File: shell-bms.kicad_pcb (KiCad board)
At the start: 4 copper layers, 128.2 x 122.2 mm, 196 parts, among them J1 Conn_01x20, J10 Conn_01x05, J11 USB_C_Receptacle_USB2.0_16P, J13 OUTSIDE LED, J2 Conn_01x20, J3 Conn_01x04, J5 USB_C_Receptacle_USB2.0_16P, J6 Conn_01x02, J7 Conn_01x02, J8 Conn_01x02, J9 Conn_01x04, Q1 NPN, Q2 HY3610P, Q3 HY3610P, Q4 BC817, Q5 BC817, Q6 BC817, Q7 BC817, Q8 HY3610P, Q9 HY3610P, SW1 SW_Push, SW2 SW_Nidec_CAS-120A1, U1 BQ76952PFBR, U2 LM5017MR, U3 STM32G431C8Tx, U4 AP2204K-5.0, U5 CH340K, U6 XC6206 - 3V3, U7 ESP-WROOM-02, U8 TJA1051T, U9 CH340K, Y1 8MHz

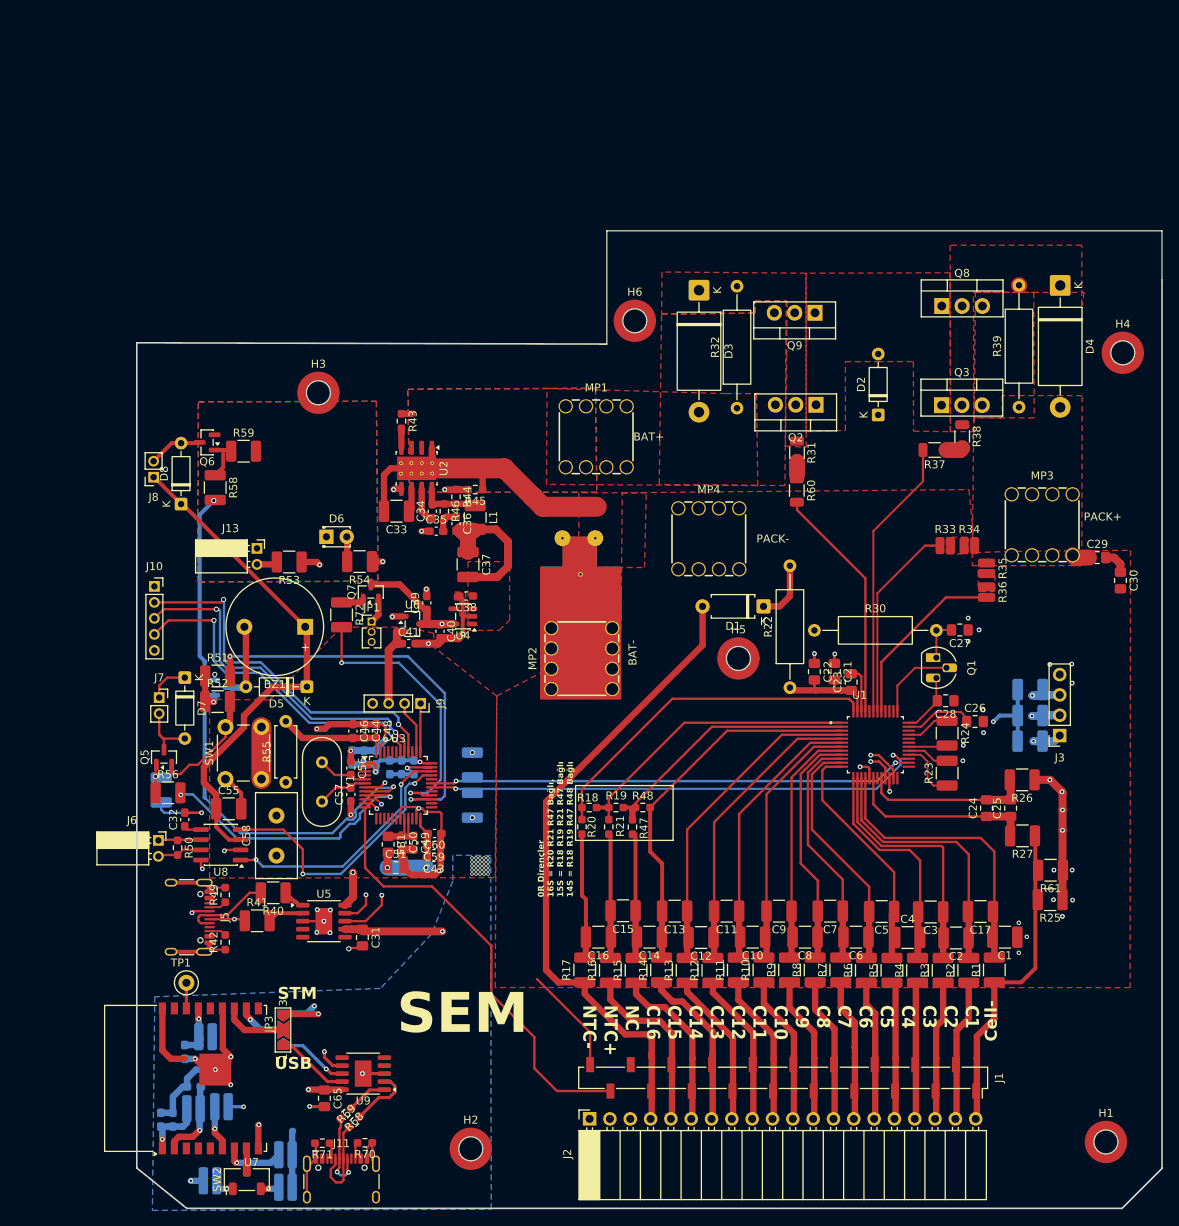
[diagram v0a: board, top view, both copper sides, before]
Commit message: BMS DONE IHOPE
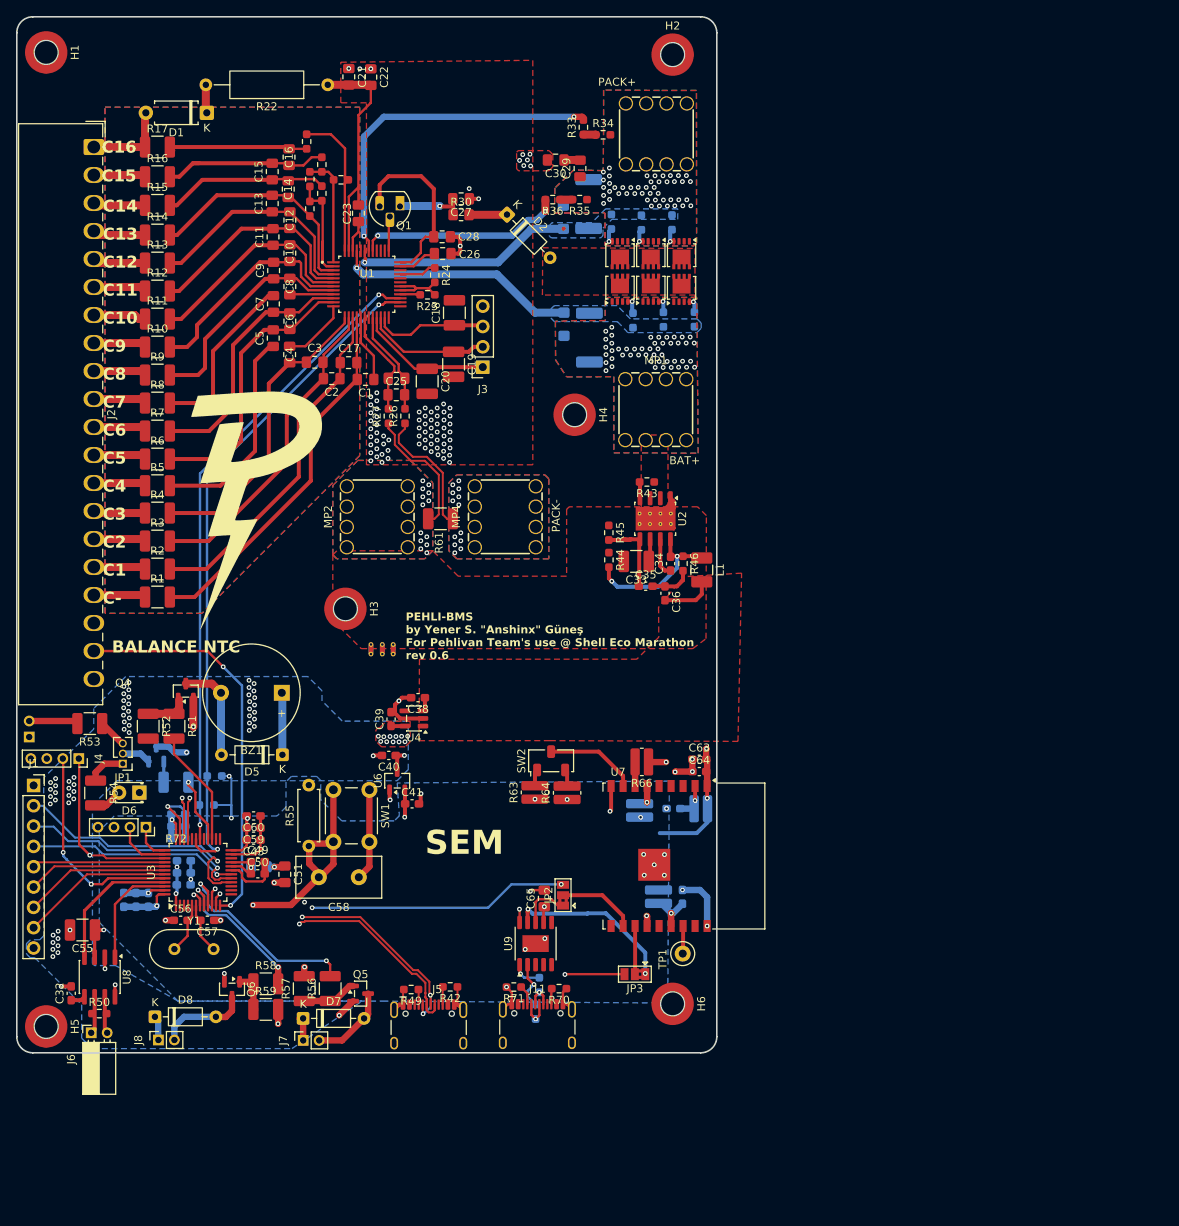
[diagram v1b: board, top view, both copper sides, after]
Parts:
- removed C31: 100nf, Capacitor_SMD:C_0805_2012Metric_Pad1.18x1.45mm_HandSolder
- removed C37: 47uF, Capacitor_SMD:C_1210_3225Metric_Pad1.33x2.70mm_HandSolder
- removed J10: Conn_01x05, Connector_PinSocket_2.00mm:PinSocket_1x05_P2.00mm_Vertical
- removed R40, R41: 22R, Resistor_SMD:R_1210_3225Metric_Pad1.30x2.65mm_HandSolder
- removed U5: CH340K, Package_SO:SSOP-10-1EP_3.9x4.9mm_P1mm_EP2.1x3.3mm
- added J4: Conn_01x04, Connector_PinSocket_2.00mm:PinSocket_1x04_P2.00mm_Vertical, F.Cu at (39.2, 113.7)
- added NT2: NetTie_2, NetTie:NetTie-2_THT_Pad0.3mm, F.Cu at (77.2, 99.5)
- added NT3: NetTie_2, NetTie:NetTie-2_THT_Pad0.3mm, F.Cu at (75.8, 99.5)
- added Q10: BUK7M27-80EX, Package_TO_SOT_SMD:LFPAK33, F.Cu at (110.7, 50.6)
- added Q11: BUK7M27-80EX, Package_TO_SOT_SMD:LFPAK33, F.Cu at (114.6, 50.6)
- added R73: 47, Resistor_SMD:R_0603_1608Metric_Pad0.98x0.95mm_HandSolder, B.Cu at (113.4, 46.7)
- C1, C10, C11, C12, C13, C14, C15, C16, C17, C2, C3, C4, C5, C6, C7, C8, C9: footprint Capacitor_SMD:C_1210_3225Metric_Pad1.33x2.70mm_HandSolder -> Capacitor_SMD:C_0805_2012Metric_Pad1.18x1.45mm_HandSolder
- C18, C19, C20, C63, C64, G***, Q4, R57, R63, R64, R66: moved to F.Cu
- C44, C46, C48, FB1, J13, Q7, R68, R69, R72: moved to B.Cu
- D3, D4: footprint Diode_THT:D_DO-201_P15.24mm_Horizontal -> Diode_SMD:D_SMF; moved to B.Cu
- J1: value Conn_01x20 -> Conn_01x09; footprint Connector_PinSocket_2.54mm:PinSocket_1x20_P2.54mm_Vertical_SMD_Pin1Right -> Connector_PinSocket_2.54mm:PinSocket_1x09_P2.54mm_Vertical
- J2: footprint Connector_PinSocket_2.54mm:PinSocket_1x20_P2.54mm_Horizontal -> Connector_Wago:Wago_734-180_1x20_P3.50mm_Horizontal
- JP2: footprint Jumper:SolderJumper-3_P2.0mm_Open_TrianglePad1.0x1.5mm_NumberLabels -> Jumper:SolderJumper-3_P1.3mm_Bridged2Bar12_Pad1.0x1.5mm; moved to F.Cu
- JP3: footprint Jumper:SolderJumper-3_P2.0mm_Open_TrianglePad1.0x1.5mm_NumberLabels -> Jumper:SolderJumper-3_P1.3mm_Bridged2Bar12_Pad1.0x1.5mm
- NT1: value NetTie_3_Tee -> NetTie_2; footprint NetTie:NetTie-3_THT_Pad0.3mm -> NetTie:NetTie-2_THT_Pad0.3mm
- Q2, Q3, Q8, Q9: value HY3610P -> BUK7M27-80EX; footprint Package_TO_SOT_THT:TO-220-3_Vertical -> Package_TO_SOT_SMD:LFPAK33
- R23, R24, R26, R27, R28, R29: footprint Resistor_SMD:R_1210_3225Metric_Pad1.30x2.65mm_HandSolder -> Resistor_SMD:R_0603_1608Metric_Pad0.98x0.95mm_HandSolder
- R25: value 1m -> 47; footprint Resistor_SMD:R_1210_3225Metric_Pad1.30x2.65mm_HandSolder -> Resistor_SMD:R_0603_1608Metric_Pad0.98x0.95mm_HandSolder; moved to B.Cu
- R30: value R -> 300; footprint Resistor_THT:R_Axial_DIN0309_L9.0mm_D3.2mm_P15.24mm_Horizontal -> Resistor_SMD:R_0805_2012Metric_Pad1.20x1.40mm_HandSolder
- R31, R37, R60: value 2k -> 47; footprint Resistor_SMD:R_1206_3216Metric -> Resistor_SMD:R_0603_1608Metric_Pad0.98x0.95mm_HandSolder; moved to B.Cu
- R32: footprint Resistor_THT:R_Axial_DIN0309_L9.0mm_D3.2mm_P15.24mm_Horizontal -> Resistor_SMD:R_2512_6332Metric_Pad1.40x3.35mm_HandSolder; moved to B.Cu
- R33, R34, R35, R36: footprint Resistor_SMD:R_0508_1220Metric_Pad1.12x2.15mm_HandSolder -> Resistor_SMD:R_0603_1608Metric_Pad0.98x0.95mm_HandSolder
- R38: value 2k -> 1M; footprint Resistor_SMD:R_1206_3216Metric -> Resistor_SMD:R_2512_6332Metric_Pad1.40x3.35mm_HandSolder; moved to B.Cu
- R39: value 1M -> 47; footprint Resistor_THT:R_Axial_DIN0309_L9.0mm_D3.2mm_P15.24mm_Horizontal -> Resistor_SMD:R_0603_1608Metric_Pad0.98x0.95mm_HandSolder; moved to B.Cu
- moved H1 190.0 mm to (35.2, 25.4), turned to -90 degrees
- moved H2 139.1 mm to (113.5, 25.7)
- moved J2 136.4 mm to (41.1, 37.3), turned to -90 degrees
- moved R17 115.9 mm to (49.1, 37.3), turned to 0 degrees
- moved R1 114.5 mm to (49.1, 93.5), turned to 0 degrees
- moved R16 114.2 mm to (49.1, 41.0), turned to 0 degrees
- moved R2 113.1 mm to (49.1, 90.0), turned to 0 degrees
- moved R15 112.8 mm to (49.1, 44.6), turned to 0 degrees
- moved R3 111.9 mm to (49.1, 86.5), turned to 0 degrees
- moved R14 111.4 mm to (49.1, 48.3), turned to 0 degrees
- moved R4 110.9 mm to (49.1, 83.0), turned to 0 degrees
- moved R13 110.5 mm to (49.1, 51.8), turned to 0 degrees
- moved R5 110.0 mm to (49.1, 79.6), turned to 0 degrees
- moved R12 109.7 mm to (49.1, 55.3), turned to 0 degrees
- moved R6 109.3 mm to (49.1, 76.3), turned to 0 degrees
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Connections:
- net /Data_Utils/RXD renamed /MCU/esp32/ESP_RX
- net /Data_Utils/TXD renamed /MCU/esp32/ESP_TX
- C29 pad 1: Net-(D4-A) -> /Protection/PACK+
- D1 pad 2: /ReaderIC/Balance-Input/B_16 -> /ReaderIC/Balance-Input/CI_16
- D3 pad 1: Net-(D3-K) -> /Protection/CHG_GATE
- D3 pad 2: /Protection/B_Pos -> /Protection/B_POS
- D4 pad 1: Net-(D4-K) -> /Protection/DSG_GATE
- D4 pad 2: Net-(D4-A) -> /Protection/PACK+
- J1 pad 1: /ReaderIC/Balance-Input/B_0 -> GND
- J1 pad 2: /ReaderIC/Balance-Input/B_1 -> /Data_Utils/PB0
- J1 pad 3: /ReaderIC/Balance-Input/B_2 -> /Data_Utils/PB1
- J1 pad 4: /ReaderIC/Balance-Input/B_3 -> /Data_Utils/PB2
- J1 pad 5: /ReaderIC/Balance-Input/B_4 -> /Data_Utils/PB3
- J1 pad 6: /ReaderIC/Balance-Input/B_5 -> /Data_Utils/PB4
- J1 pad 7: /ReaderIC/Balance-Input/B_6 -> /Data_Utils/PB5
- J1 pad 8: /ReaderIC/Balance-Input/B_7 -> /Data_Utils/PB6
- J1 pad 9: /ReaderIC/Balance-Input/B_8 -> +5V
- J2 pad 1: /ReaderIC/Balance-Input/B_0 -> /ReaderIC/Balance-Input/CI_16
- J2 pad 10: /ReaderIC/Balance-Input/B_9 -> /ReaderIC/Balance-Input/CI_7
- J2 pad 11: /ReaderIC/Balance-Input/B_10 -> /ReaderIC/Balance-Input/CI_6
- J2 pad 12: /ReaderIC/Balance-Input/B_11 -> /ReaderIC/Balance-Input/CI_5
- J2 pad 13: /ReaderIC/Balance-Input/B_12 -> /ReaderIC/Balance-Input/CI_4
- J2 pad 14: /ReaderIC/Balance-Input/B_13 -> /ReaderIC/Balance-Input/CI_3
- J2 pad 15: /ReaderIC/Balance-Input/B_14 -> /ReaderIC/Balance-Input/CI_2
- J2 pad 16: /ReaderIC/Balance-Input/B_15 -> /ReaderIC/Balance-Input/CI_1
- J2 pad 17: /ReaderIC/Balance-Input/B_16 -> /ReaderIC/Balance-Input/CI_0
- J2 pad 19: unconnected-(J2-Pin_19-Pad19) -> /MCU/NTC
- J2 pad 2: /ReaderIC/Balance-Input/B_1 -> /ReaderIC/Balance-Input/CI_15
- J2 pad 20: unconnected-(J2-Pin_20-Pad20) -> GND
- J2 pad 3: /ReaderIC/Balance-Input/B_2 -> /ReaderIC/Balance-Input/CI_14
- J2 pad 4: /ReaderIC/Balance-Input/B_3 -> /ReaderIC/Balance-Input/CI_13
- J2 pad 5: /ReaderIC/Balance-Input/B_4 -> /ReaderIC/Balance-Input/CI_12
- J2 pad 6: /ReaderIC/Balance-Input/B_5 -> /ReaderIC/Balance-Input/CI_11
- J2 pad 7: /ReaderIC/Balance-Input/B_6 -> /ReaderIC/Balance-Input/CI_10
- J2 pad 8: /ReaderIC/Balance-Input/B_7 -> /ReaderIC/Balance-Input/CI_9
- J2 pad 9: /ReaderIC/Balance-Input/B_8 -> /ReaderIC/Balance-Input/CI_8
- J5 pad A6: Net-(J5-D+-PadA6) -> /Data_Utils/USB+
- J5 pad A7: Net-(J5-D--PadA7) -> /Data_Utils/USB-
- J5 pad B6: Net-(J5-D+-PadA6) -> /Data_Utils/USB+
- J5 pad B7: Net-(J5-D--PadA7) -> /Data_Utils/USB-
- MP1 pad 1: /Protection/B_Pos -> /Protection/B_POS
- MP1 pad 2: /Protection/B_Pos -> /Protection/B_POS
- MP1 pad 3: /Protection/B_Pos -> /Protection/B_POS
- MP1 pad 4: /Protection/B_Pos -> /Protection/B_POS
- MP1 pad 5: /Protection/B_Pos -> /Protection/B_POS
- MP1 pad 6: /Protection/B_Pos -> /Protection/B_POS
- MP1 pad 7: /Protection/B_Pos -> /Protection/B_POS
- MP1 pad 8: /Protection/B_Pos -> /Protection/B_POS
- MP2 pad 1: Net-(MP2-Pad1) -> GNDPWR
- MP2 pad 2: Net-(MP2-Pad1) -> GNDPWR
- MP2 pad 3: Net-(MP2-Pad1) -> GNDPWR
- MP2 pad 4: Net-(MP2-Pad1) -> GNDPWR
- MP2 pad 5: Net-(MP2-Pad1) -> GNDPWR
- MP2 pad 6: Net-(MP2-Pad1) -> GNDPWR
- MP2 pad 7: Net-(MP2-Pad1) -> GNDPWR
- MP2 pad 8: Net-(MP2-Pad1) -> GNDPWR
- MP3 pad 1: Net-(D4-A) -> /Protection/PACK+
- MP3 pad 2: Net-(D4-A) -> /Protection/PACK+
- MP3 pad 3: Net-(D4-A) -> /Protection/PACK+
- MP3 pad 4: Net-(D4-A) -> /Protection/PACK+
- MP3 pad 5: Net-(D4-A) -> /Protection/PACK+
- MP3 pad 6: Net-(D4-A) -> /Protection/PACK+
- MP3 pad 7: Net-(D4-A) -> /Protection/PACK+
- MP3 pad 8: Net-(D4-A) -> /Protection/PACK+
- NT1 pad 1: GND -> GNDPWR
- NT1 pad 2: GNDPWR -> GND
- Q2 pad 1: /Protection/CD -> /Protection/PACK+
- Q2 pad 2: Net-(D3-K) -> /Protection/PACK+
- Q2 pad 3: /Protection/B_Pos -> /Protection/PACK+
- Q3 pad 1: /Protection/CD -> /Protection/B_POS
- Q3 pad 2: Net-(D4-K) -> /Protection/B_POS
- Q3 pad 3: Net-(D4-A) -> /Protection/B_POS
- Q7 pad 2: Net-(JP1-A) -> Net-(JP1-C)
- Q8 pad 1: /Protection/CD -> /Protection/B_POS
- Q8 pad 2: Net-(D4-K) -> /Protection/B_POS
- Q8 pad 3: Net-(D4-A) -> /Protection/B_POS
- Q9 pad 1: /Protection/CD -> /Protection/B_POS
- Q9 pad 2: Net-(D3-K) -> /Protection/B_POS
- Q9 pad 3: /Protection/B_Pos -> /Protection/B_POS
- R1 pad 1: /ReaderIC/Balance-Input/B_0 -> /ReaderIC/Balance-Input/CI_0
- R10 pad 1: /ReaderIC/Balance-Input/B_9 -> /ReaderIC/Balance-Input/CI_9
- R11 pad 1: /ReaderIC/Balance-Input/B_10 -> /ReaderIC/Balance-Input/CI_10
- R12 pad 1: /ReaderIC/Balance-Input/B_11 -> /ReaderIC/Balance-Input/CI_11
- R13 pad 1: /ReaderIC/Balance-Input/B_12 -> /ReaderIC/Balance-Input/CI_12
- R14 pad 1: /ReaderIC/Balance-Input/B_13 -> /ReaderIC/Balance-Input/CI_13
- R15 pad 1: /ReaderIC/Balance-Input/B_14 -> /ReaderIC/Balance-Input/CI_14
- R16 pad 1: /ReaderIC/Balance-Input/B_15 -> /ReaderIC/Balance-Input/CI_15
- R17 pad 1: /ReaderIC/Balance-Input/B_16 -> /ReaderIC/Balance-Input/CI_16
- R2 pad 1: /ReaderIC/Balance-Input/B_1 -> /ReaderIC/Balance-Input/CI_1
- R25 pad 1: GNDPWR -> /Protection/CHG_GATE
- R25 pad 2: /ReaderIC/Balance-Input/B_0 -> Net-(Q8-G)
- R27 pad 1: /ReaderIC/Balance-Input/B_0 -> GNDPWR
- R28 pad 1: /MCU/IC_SDA -> +3V3
- R28 pad 2: +3V3 -> /MCU/IC_SCL
- R29 pad 1: +3V3 -> /MCU/IC_SDA
- R29 pad 2: /MCU/IC_SCL -> +3V3
- R3 pad 1: /ReaderIC/Balance-Input/B_2 -> /ReaderIC/Balance-Input/CI_2
- R31 pad 1: Net-(D3-K) -> /Protection/CHG_GATE
- R31 pad 2: Net-(R31-Pad2) -> Net-(Q3-G)
- R32 pad 1: /Protection/B_Pos -> /Protection/B_POS
- R32 pad 2: Net-(D3-K) -> /Protection/CHG_GATE
- R33 pad 1: /Protection/PACK -> Net-(R33-Pad1)
- R33 pad 2: Net-(R33-Pad2) -> /Protection/PACK
- R34 pad 1: Net-(R33-Pad2) -> Net-(R33-Pad1)
- R34 pad 2: Net-(D4-A) -> /Protection/PACK+
- R35 pad 1: Net-(D4-A) -> /Protection/PACK+
- R37 pad 1: Net-(R37-Pad1) -> /Protection/CHG_GATE
- R37 pad 2: /Protection/DSG -> Net-(Q9-G)
- R38 pad 1: Net-(D4-K) -> /Protection/PACK+
- R38 pad 2: Net-(R37-Pad1) -> /Protection/DSG_GATE
- R39 pad 1: Net-(D4-A) -> /Protection/DSG_GATE
- R39 pad 2: Net-(D4-K) -> Net-(Q2-G)
- R4 pad 1: /ReaderIC/Balance-Input/B_3 -> /ReaderIC/Balance-Input/CI_3
- R43 pad 1: /Protection/B_Pos -> /Protection/B_POS
- R5 pad 1: /ReaderIC/Balance-Input/B_4 -> /ReaderIC/Balance-Input/CI_4
- R53 pad 1: Net-(JP1-C) -> Net-(JP1-B)
- R54 pad 1: Net-(JP1-B) -> Net-(JP1-A)
- R6 pad 1: /ReaderIC/Balance-Input/B_5 -> /ReaderIC/Balance-Input/CI_5
- R60 pad 1: Net-(R31-Pad2) -> /Protection/DSG_GATE
- R60 pad 2: /Protection/CHG -> Net-(Q10-G)
- R61 pad 2: /ReaderIC/Balance-Input/B_0 -> GNDPWR
- R7 pad 1: /ReaderIC/Balance-Input/B_6 -> /ReaderIC/Balance-Input/CI_6
- R8 pad 1: /ReaderIC/Balance-Input/B_7 -> /ReaderIC/Balance-Input/CI_7
- R9 pad 1: /ReaderIC/Balance-Input/B_8 -> /ReaderIC/Balance-Input/CI_8
- U1 pad 43: /Protection/DSG -> /Protection/DSG_GATE
- U1 pad 45: /Protection/CHG -> /Protection/CHG_GATE
- U2 pad 2: /Protection/B_Pos -> /Protection/B_POS
- U2 pad 3: /Protection/B_Pos -> /Protection/B_POS
- U3 pad 16: unconnected-(U3-PB0-Pad16) -> /Data_Utils/PB0
- U3 pad 17: unconnected-(U3-PB1-Pad17) -> /Data_Utils/PB1
- U3 pad 18: unconnected-(U3-PB2-Pad18) -> /Data_Utils/PB2
- U3 pad 33: /Data_Utils/CAN_RX -> /Data_Utils/USB+
- U3 pad 34: /Data_Utils/CAN_TX -> /Data_Utils/USB-
- U3 pad 39: unconnected-(U3-PA15-Pad39) -> /MCU/I2C_SCL
- U3 pad 43: unconnected-(U3-PB6-Pad43) -> /Data_Utils/PB6
- U3 pad 44: unconnected-(U3-PB7-Pad44) -> /MCU/I2C_SDA
- U3 pad 45: unconnected-(U3-PB8-Pad45) -> /Data_Utils/CAN_RX
- U3 pad 46: unconnected-(U3-PB9-Pad46) -> /Data_Utils/CAN_TX
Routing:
- net +5V: track 123.9 -> 30.1 mm, vias 1 -> 68
- net GND: track 188.2 -> 105.7 mm, vias 30 -> 38
- net /ReaderIC/Balance-Input/B_16: track 81.9 -> 0.00 mm
- net /Data_Utils/USB-: track 4.54 -> 60.3 mm, vias 0 -> 4
- net /Data_Utils/USB+: track 2.79 -> 57.7 mm, vias 0 -> 2
- net /Data_Utils/FAN2: track 70.7 -> 19.4 mm
- net /ReaderIC/Balance-Input/B_0: track 40.9 -> 0.00 mm
- net +3V3: track 122.2 -> 82.5 mm, vias 36 -> 14
- net /Data_Utils/BUZZER: track 51.0 -> 14.5 mm, vias 2 -> 0
- net /Protection/DSG: track 35.2 -> 0.00 mm
- net /Data_Utils/PB0: track 0.00 -> 32.6 mm, vias 0 -> 1
- net GNDPWR: track 95.4 -> 63.5 mm, vias 26 -> 103
- net /Protection/CHG_GATE: track 0.00 -> 30.4 mm, vias 0 -> 1
- net /Protection/CHG: track 30.1 -> 0.00 mm
- net /Data_Utils/PB3: track 46.0 -> 16.6 mm, vias 2 -> 0
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- added copper zone on B.Cu, net (none)
- added copper zone on F.Cu, net (none)
- added copper zone on In1.Cu, net (none)
- added copper zone on In2.Cu, net (none)
- added copper zone on In2.Cu, net +3V3
- added copper zone on B.Cu, net +5V
- added copper zone on F.Cu, net +5V
- added copper zone on In2.Cu, net +5V
- added copper zone on B.Cu, net /Protection/B_POS
- added copper zone on F.Cu, net /Protection/B_POS
- added copper zone on In1.Cu, net /Protection/B_POS
- added copper zone on In2.Cu, net /Protection/B_POS
- added copper zone on In1.Cu, net /Protection/CD
- added copper zone on In2.Cu, net /Protection/CD
- added copper zone on B.Cu, net /Protection/CHG_GATE
- added copper zone on B.Cu, net /Protection/DSG_GATE
- added copper zone on B.Cu, net /Protection/PACK+
- added copper zone on F.Cu, net /Protection/PACK+
- added copper zone on In1.Cu, net /Protection/PACK+
- added copper zone on In2.Cu, net /Protection/PACK+
- added copper zone on B.Cu, net GNDPWR
- added copper zone on In2.Cu, net GNDPWR
- removed copper zone on F.Cu, net +3V3
- removed copper zone on B.Cu, net /Protection/B_Pos
- removed copper zone on F.Cu, net /Protection/B_Pos
- removed copper zone on In1.Cu, net /Protection/B_Pos
- removed copper zone on B.Cu, net GND
- removed copper zone on F.Cu, net GND
- removed copper zone on In2.Cu, net GND
- removed copper zone on F.Cu, net Net-(D3-K)
- removed copper zone on F.Cu, net Net-(D4-A)
- removed copper zone on F.Cu, net Net-(D4-K)
- removed copper zone on F.Cu, net Net-(R33-Pad2)
- removed copper zone on F.Cu, net Net-(R35-Pad2)
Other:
- board size 128.2 x 122.2 mm -> 87.5 x 129.5 mm
- board text added: "BALANCE NTC"
- board text added: "C-"
- board text added: "C1"
- board text added: "C10"
- board text added: "C11"
- board text added: "C12"
- board text added: "C13"
- board text added: "C14"
- board text added: "C15"
- board text added: "C16"
- board text added: "C2"
- board text added: "C3"
- board text added: "C4"
- board text added: "C5"
- board text added: "C6"
- board text added: "C7"
- board text added: "C8"
- board text added: "C9"
- board text added: "PACK-"
- board text added: "PEHLI-BMS by Yener S. {dblquote}Anshinx{dblquote} Güneş For Pehlivan Team's use @ Shell Eco Marathon rev 0.6"
- board text added: "R61"
- board text added: "Takma listesi: 16S: R20 R21 R47 15S: R18 R21 R47 14S: R18 R19 R47 13S: R18 R19 R48"
- board text removed: "0R Dirençler 16S = R20 R21 R47 Bağlı, 15S = R18 R19 R21 R47 Bağlı 14S = R18 R19 R47 R48 Bağlı"
- board text removed: "16S - 15S - 14S ALL IN ONE BATTERY MANAGEMENT SYSTEM"
- board text removed: "C1 C2 C3 C4 C5 C6 C7 C8 C9 C10 C11 C12 C13 C14 C15 C16 NC NTC+ NTC-"
- board text removed: "Cell-"
- board text removed: "DESIGNED BY ANSHINX FOR PEHLIVAN TEAM"
- board text removed: "PACK+"
- board text removed: "PEHLIBMS v0.3"
- board text removed: "STM"
- board text removed: "USB"
